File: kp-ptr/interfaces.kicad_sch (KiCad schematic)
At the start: 20 parts, among them IC2 E22-900M22S, J4 USB_C_Receptacle_USB2.0, J5 u.fl, U11 USBLC6-2SC6, U12 NL27WZU04DBVT1G, U13 W25Q256

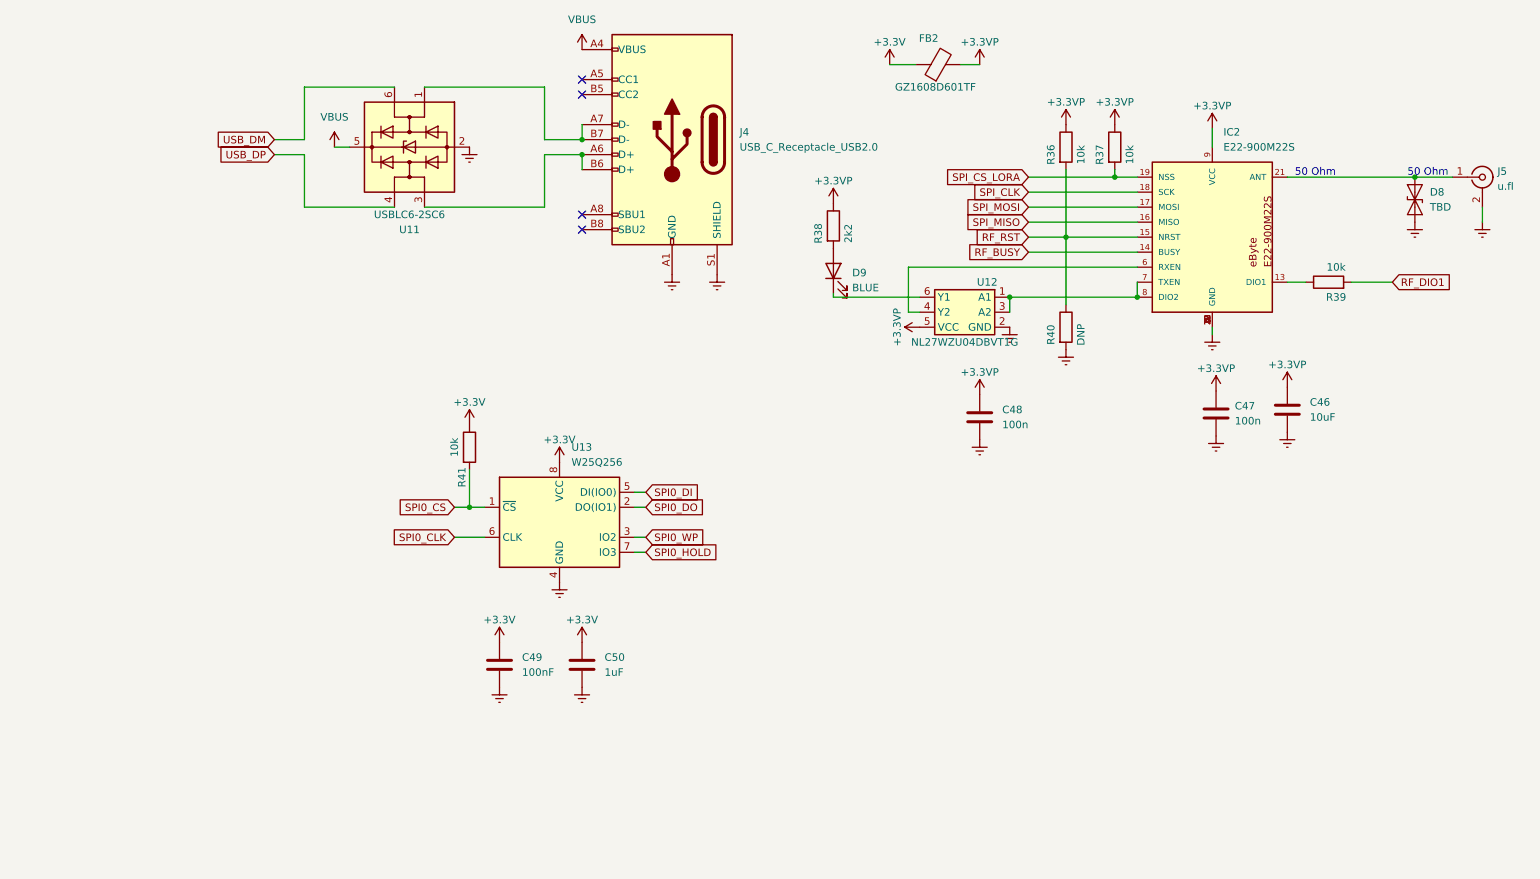
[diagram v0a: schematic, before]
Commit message: Release v1
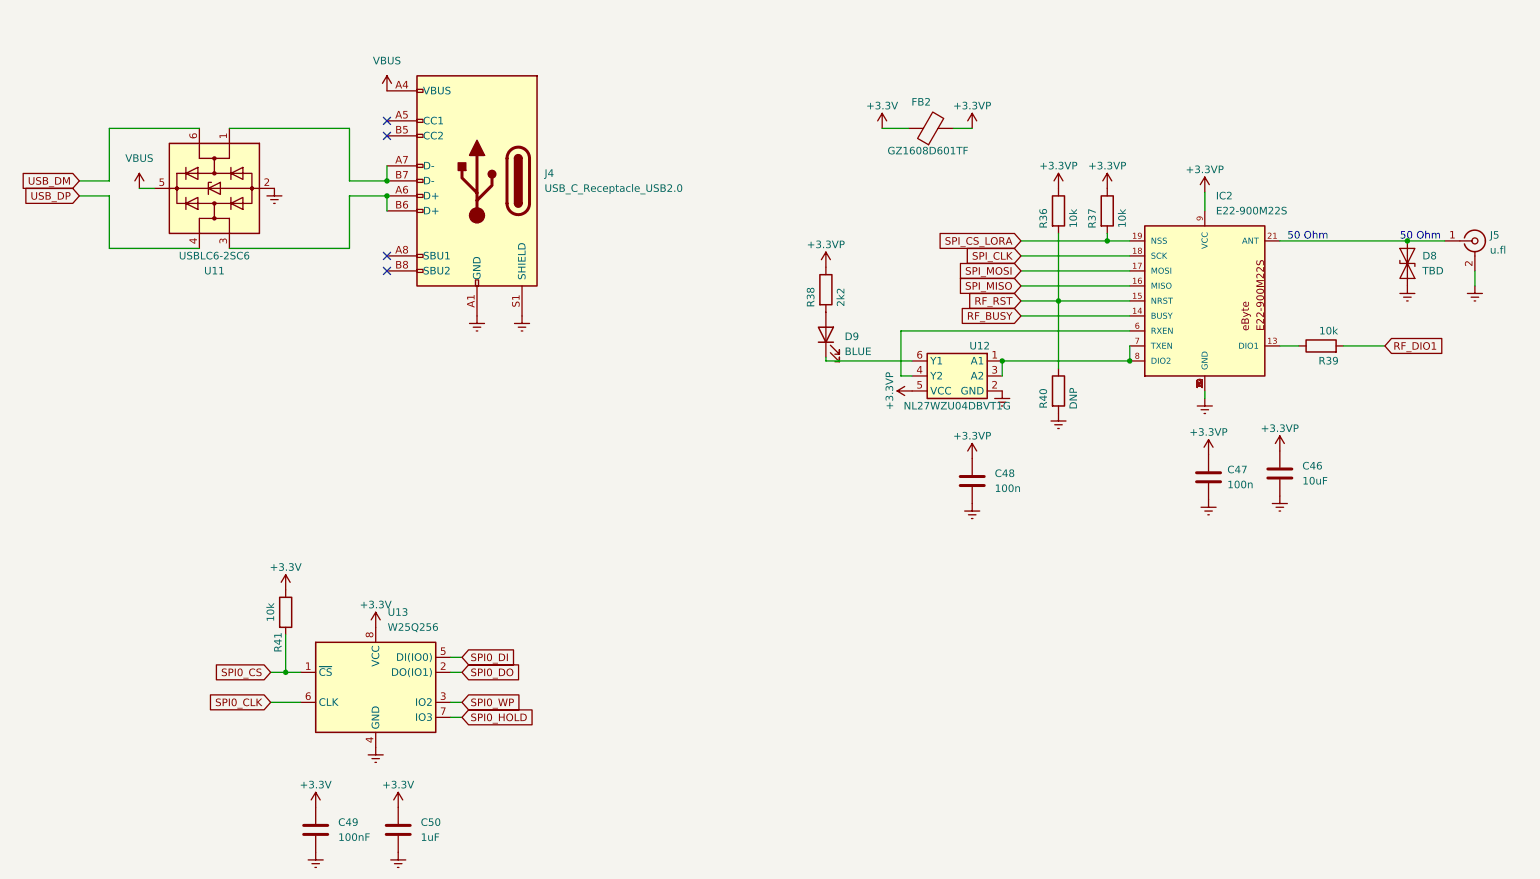
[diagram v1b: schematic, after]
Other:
- company: (none) -> Polskie Towarzystwo Rakietowe
- title: (none) -> KP-PTR
- moved on the sheet: C46, C47, C48, C49, C50, D8, D9, FB2, IC2, J4, J5, R36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
